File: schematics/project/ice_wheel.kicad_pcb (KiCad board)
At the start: 2 copper layers, 16 parts, among them Q1 BSS123, U1 OPA320xxDBV, U1 Teensy4.1, U2 PropShieldMotionSens, U3 OPA320xxDBV

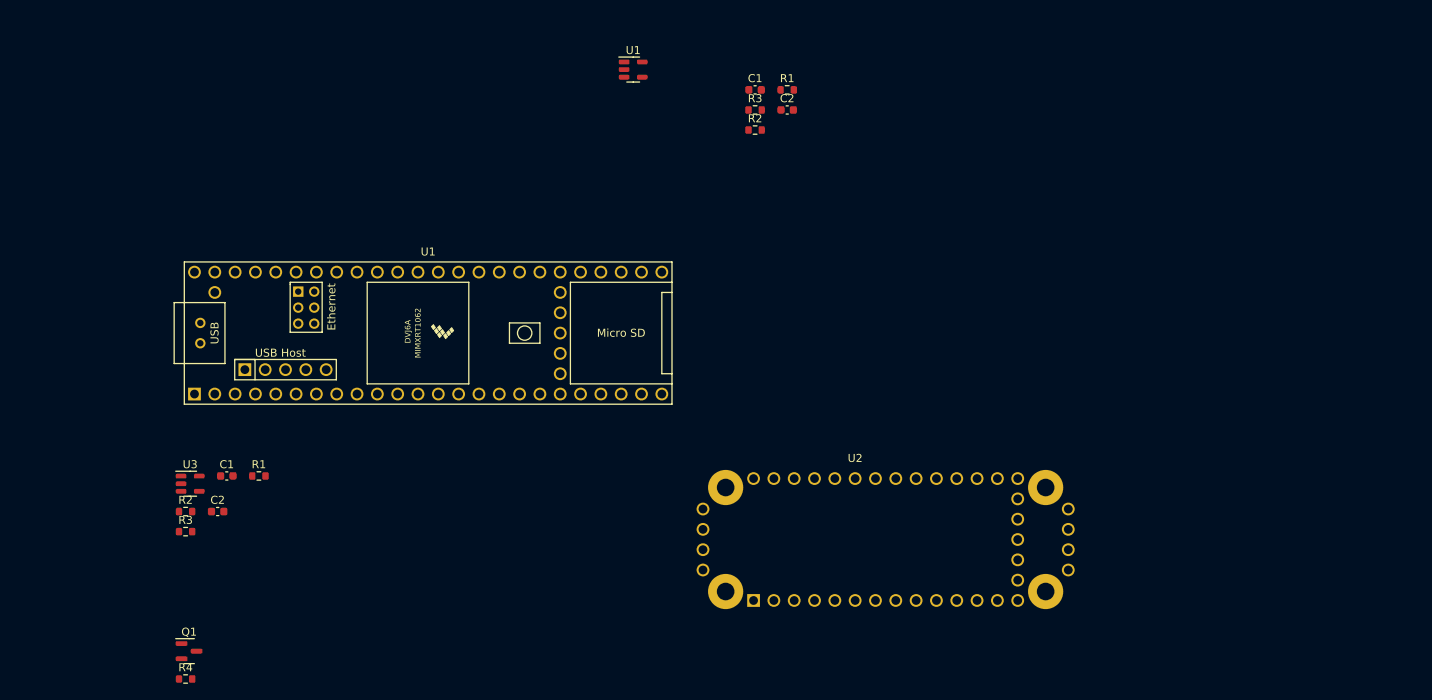
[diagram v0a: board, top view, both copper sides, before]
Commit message: some progress, dust slowly clears
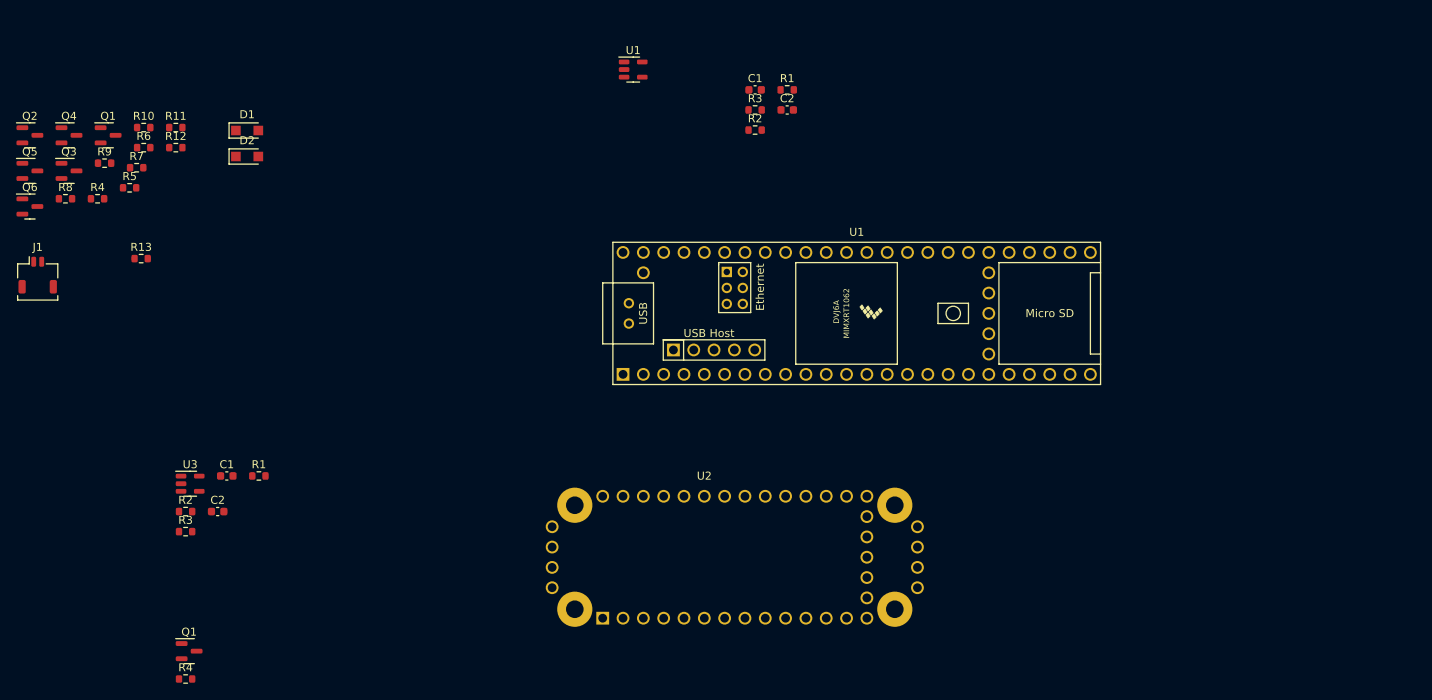
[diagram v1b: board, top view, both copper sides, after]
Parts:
- added D1: PMEG40T20ER, Diode_SMD:Nexperia_CFP3_SOD-123W, F.Cu at (61.0, 94.0)
- added D2: PMEG40T20ER, Diode_SMD:Nexperia_CFP3_SOD-123W, F.Cu at (61.0, 97.2)
- added J1: Conn_01x02, Connector_JST:JST_SHL_SM02B-SHLS-TF_1x02-1MP_P1.00mm_Horizontal, F.Cu at (34.8, 112.1)
- added Q1: BSS123, Package_TO_SOT_SMD:SOT-23, F.Cu at (43.6, 94.6)
- added Q2: BSS123, Package_TO_SOT_SMD:SOT-23, F.Cu at (33.8, 94.6)
- added Q3: BSS123, Package_TO_SOT_SMD:SOT-23, F.Cu at (38.7, 99.0)
- added Q4: BSS123, Package_TO_SOT_SMD:SOT-23, F.Cu at (38.7, 94.6)
- added Q5: BSS123, Package_TO_SOT_SMD:SOT-23, F.Cu at (33.8, 99.0)
- added Q6: BSS123, Package_TO_SOT_SMD:SOT-23, F.Cu at (33.8, 103.5)
- added R10: 1k, Resistor_SMD:R_0603_1608Metric, F.Cu at (48.0, 93.6)
- added R11: 1k, Resistor_SMD:R_0603_1608Metric, F.Cu at (52.0, 93.6)
- added R12: 1k, Resistor_SMD:R_0603_1608Metric, F.Cu at (52.0, 96.1)
- added R13: R, Resistor_SMD:R_0603_1608Metric, F.Cu at (47.7, 110.0)
- added R4: R, Resistor_SMD:R_0603_1608Metric, F.Cu at (42.3, 102.5)
- added R5: R, Resistor_SMD:R_0603_1608Metric, F.Cu at (46.3, 101.1)
- added R6: R, Resistor_SMD:R_0603_1608Metric, F.Cu at (48.0, 96.1)
- added R7: 1k, Resistor_SMD:R_0603_1608Metric, F.Cu at (47.2, 98.6)
- added R8: 1k, Resistor_SMD:R_0603_1608Metric, F.Cu at (38.3, 102.5)
- added R9: 1k, Resistor_SMD:R_0603_1608Metric, F.Cu at (43.1, 98.1)
- moved U1 53.6 mm to (137.2, 116.8)
- moved U2 19.0 mm to (105.4, 154.9)
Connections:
- net /Motor Controller/Dig2Analog/SetSpeed_Analog renamed /Motor Controller/throttle_IN
- U1 pad 1: unconnected-(U1-Pad1) -> GND
- U1 pad 12: /Teensy/CS -> /Prop Shield/CS
- U1 pad 13: /Teensy/MOSI -> /Prop Shield/MOSI
- U1 pad 14: /Teensy/MISO -> /Prop Shield/MISO
- U1 pad 35: /Teensy/SCK -> /Prop Shield/SCK
- U1 pad 36: unconnected-(U1-Pad36) -> /Misc/footpad_a 
- U1 pad 4: /Teensy/IRQ -> /Prop Shield/IRQ
- U1 pad 40: /Teensy/SDA -> /Prop Shield/SDA
- U1 pad 41: /Teensy/SCL -> /Prop Shield/SCL
- U1 pad 46: unconnected-(U1-Pad46) -> +3V3
- U1 pad 48: unconnected-(U1-Pad48) -> +5P
- U1 pad 49: unconnected-(U1-Pad49) -> +5F
- U1 pad 64: unconnected-(U1-Pad64) -> GND

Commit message: small progress, angsthasen
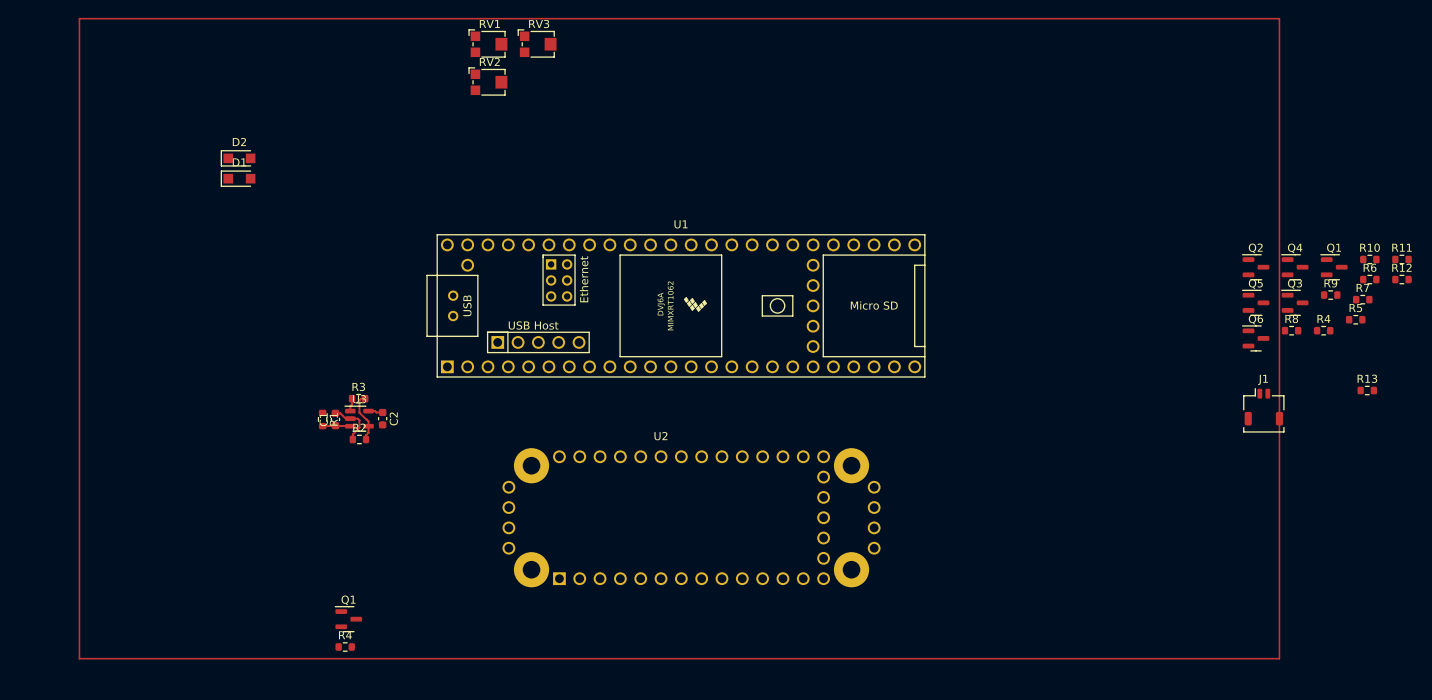
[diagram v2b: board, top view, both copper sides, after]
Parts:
- removed the C1 at (58.4, 137.2)
- removed the C1 at (124.5, 88.9)
- removed the C2 at (57.3, 141.6)
- removed the C2 at (128.5, 91.4)
- removed the R1 at (128.5, 88.9)
- removed the R1 at (62.4, 137.2)
- removed the R2 at (53.3, 141.6)
- removed the R2 at (124.5, 93.9)
- removed the R3 at (53.3, 144.1)
- removed the R3 at (124.5, 91.4)
- removed the U1 at (109.2, 86.4)
- added C1: C, Capacitor_SMD:C_0603_1608Metric, F.Cu at (72.0, 130.1)
- added C2: 100nF 10V, Capacitor_SMD:C_0603_1608Metric, F.Cu at (77.9, 130.0)
- added R1: R, Resistor_SMD:R_0603_1608Metric, F.Cu at (70.4, 130.1)
- added R2: R, Resistor_SMD:R_0603_1608Metric, F.Cu at (75.0, 132.6)
- added R3: R, Resistor_SMD:R_0603_1608Metric, F.Cu at (74.9, 127.5)
- added RV1: TC33X-1-203E, Potentiometer_SMD:Potentiometer_Bourns_TC33X_Vertical, F.Cu at (91.3, 83.2)
- added RV2: TC33X-1-203E, Potentiometer_SMD:Potentiometer_Bourns_TC33X_Vertical, F.Cu at (91.3, 88.0)
- added RV3: TC33X-1-203E, Potentiometer_SMD:Potentiometer_Bourns_TC33X_Vertical, F.Cu at (97.5, 83.2)
- R4, R5, R6: value R -> 1k
- moved J1 154.1 mm to (188.1, 128.6)
- moved Q3 154.1 mm to (192.0, 115.5)
- moved Q4 154.1 mm to (192.0, 111.1)
- moved R10 154.1 mm to (201.3, 110.1)
- moved R6 154.1 mm to (201.3, 112.6)
- moved R8 154.1 mm to (191.5, 119.0)
- moved Q1 154.1 mm to (196.8, 111.1)
- moved Q2 154.1 mm to (187.1, 111.1)
- moved Q5 154.1 mm to (187.1, 115.5)
- moved Q6 154.1 mm to (187.1, 120.0)
- moved R11 154.1 mm to (205.3, 110.1)
- moved R12 154.1 mm to (205.3, 112.6)
- moved R13 154.1 mm to (201.0, 126.5)
- moved R4 154.1 mm to (195.5, 119.0)
- moved R5 154.1 mm to (199.5, 117.6)
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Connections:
- U1 pad 15: unconnected-(U1-Pad15) -> +3V3
- U1 pad 34: unconnected-(U1-Pad34) -> GND
- U1 pad 47: unconnected-(U1-Pad47) -> GND
- U1 pad 52: unconnected-(U1-Pad52) -> GND
- U1 pad 58: unconnected-(U1-Pad58) -> GND
- U1 pad 59: unconnected-(U1-Pad59) -> GND
- U2 pad 27: unconnected-(U2-Pad27) -> /Misc/AGND
- U2 pad 33: unconnected-(U2-Pad33) -> /Misc/AudioIN
- U2 pad 39: unconnected-(U2-Pad39) -> /Misc/Speaker+
- U2 pad 40: unconnected-(U2-Pad40) -> /Misc/Speaker-
- U2 pad 41: unconnected-(U2-Pad41) -> /Misc/5V_Speaker
- U2 pad 7: unconnected-(U2-Pad7) -> /Misc/AMP_EN
- U3 pad 1: /Motor Controller/throttle_IN -> /Motor Controller/throttle_a
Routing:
- net Net-(R2-Pad2): track 0.00 -> 6.34 mm
- net GND: track 0.00 -> 6.10 mm
- net Net-(C1-Pad1): track 0.00 -> 3.47 mm
- net +5V: track 0.00 -> 1.83 mm
- net /Motor Controller/throttle_a: track 0.00 -> 1.64 mm
